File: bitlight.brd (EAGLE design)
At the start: 50.8 x 33 mm, 34 parts, among them Q1 SI4126DY-T1-GE3, Q2 FDC6330L, U1 TLV521DCKT, U2 NCP500SN33, U3 MCP73833

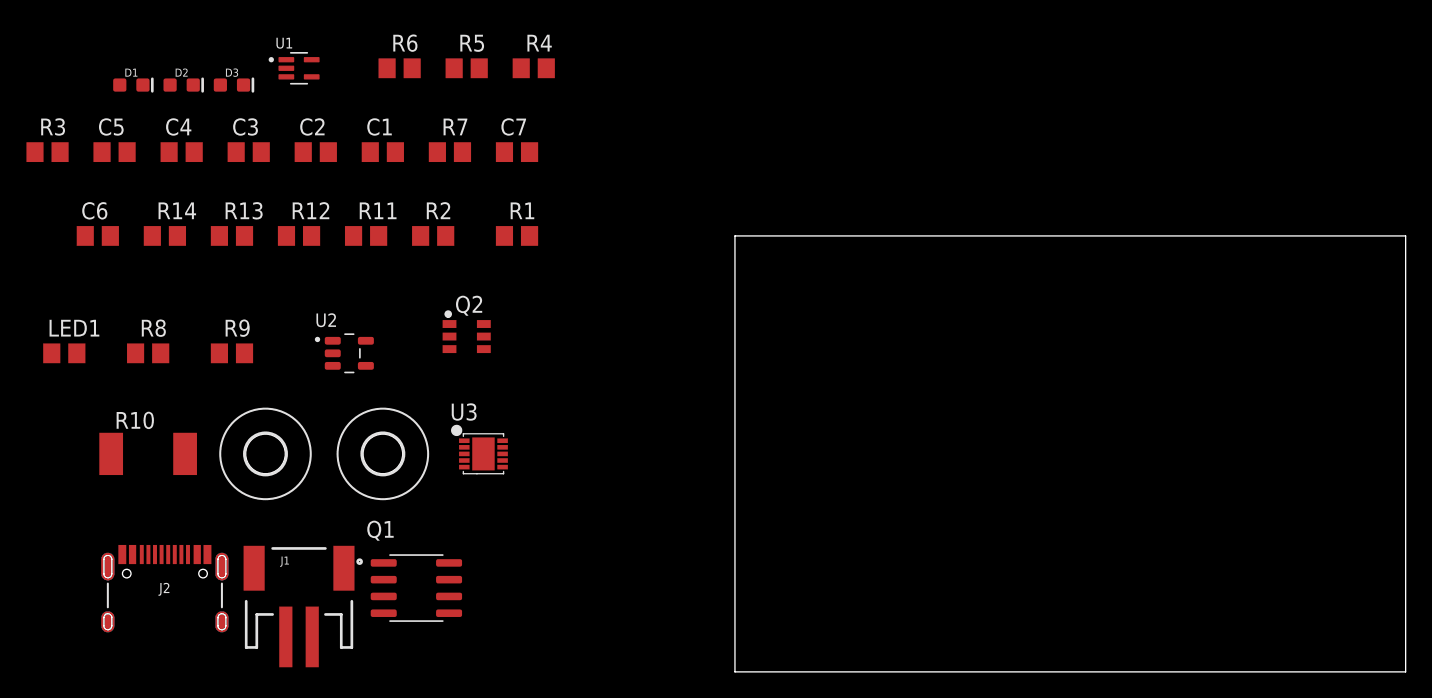
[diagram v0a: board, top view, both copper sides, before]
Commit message: final design
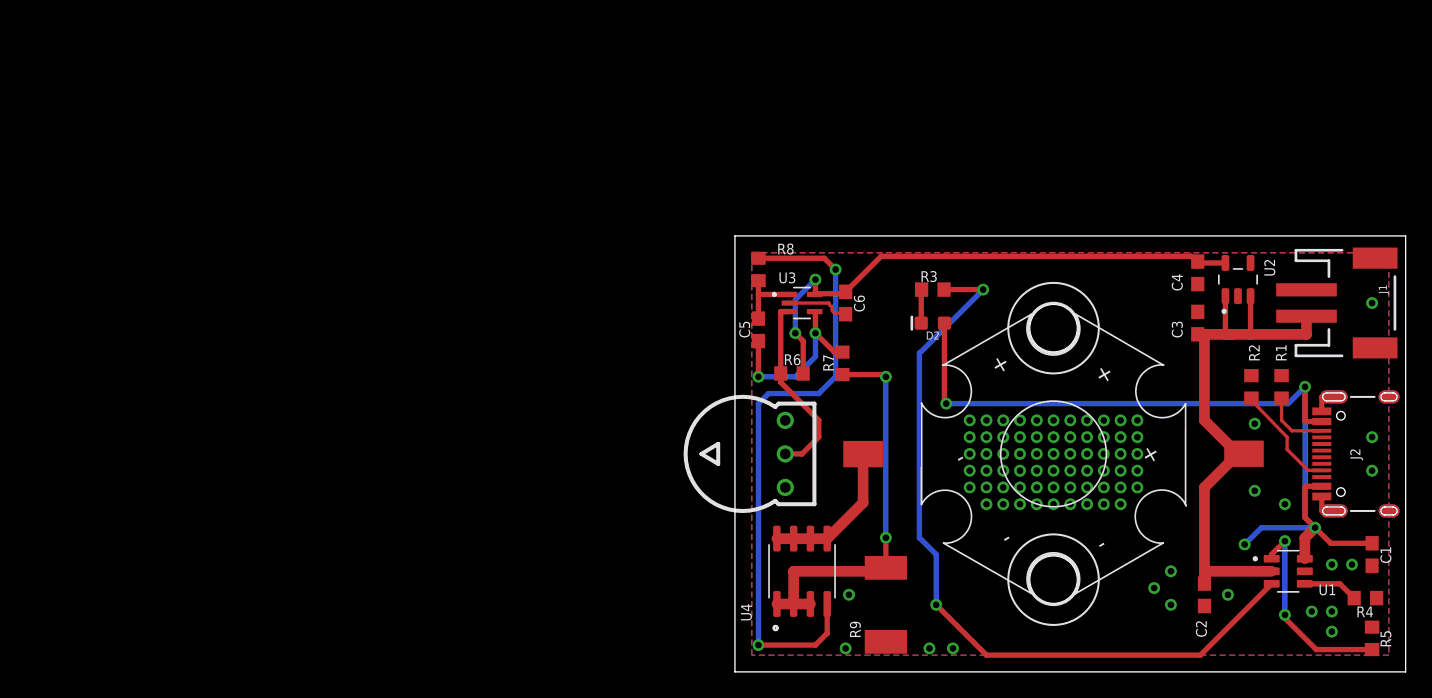
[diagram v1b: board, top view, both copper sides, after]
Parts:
- removed C7: 0.1u, rcl:C0805
- removed D3: Yellow, SparkFun-LED:LED-0603
- removed LED1: LED, rcl:C0805
- removed Q1: SI4126DY-T1-GE3, SI4126DY-T1-GE3:SOIC127P600X175-8N
- removed Q2: FDC6330L, FDC6330L:SOT95P280X110-6N
- removed R10: 0.5, rcl:R2512
- removed R11, R12, R14: 1k, rcl:R0805
- removed R13: 10k, rcl:R0805
- added P1: 3352T-1-105, 3352T-1:3352T-1
- added U4: SI4126DY-T1-GE3, SI4126DY-T1-GE3:SOIC127P600X175-8N
- C1, C2, C3, C4, C6: device rcl:C0805 -> rcl:C0603
- C5: value 1n -> 0.1u; device rcl:C0805 -> rcl:C0603
- D1: value RED -> 3W-AL-PCB; device SparkFun-LED:LED-0603 -> 3W-AL-PCB:AL-PCB-20MM
- H1, H2: value MOUNT-HOLE3.0 -> MOUNT-HOLE3.6; device holes:3,0 -> holes:3,6
- R1, R2, R3: device rcl:R0805 -> rcl:R0603
- R4: value 1k -> 680; device rcl:R0805 -> rcl:R0603
- R5: value 1k -> 10k; device rcl:R0805 -> rcl:R0603
- R6: value 1k -> 7.5M; device rcl:R0805 -> rcl:R0603
- R7: value 10k -> 1k; device rcl:R0805 -> rcl:R0603
- R8: value 7.5M -> 1k; device rcl:R0805 -> rcl:R0603
- R9: value 1M-pot -> 0.5; device rcl:R0805 -> rcl:R2512
- U1: value TLV521DCKT -> BQ21040DBVT; device TLV521DCKT:SOT65P210X110-5N -> BQ21040DBVT:SOT95P280X145-6N
- U3: value MCP73833 -> TLV521DCKT; device SparkFun-IC-Power:DFN-10 -> TLV521DCKT:SOT65P210X110-5N
- moved J2 88.0 mm to (44.5, 16.5), turned to 90 degrees
- moved U1 84.1 mm to (41.9, 7.62)
- moved J1 82.9 mm to (47.0, 27.9), turned to 270 degrees
- moved R5 81.0 mm to (48.3, 2.54), turned to 270 degrees
- moved C1 80.9 mm to (48.3, 8.89), turned to 270 degrees
- moved C4 77.5 mm to (35.1, 30.2), turned to 270 degrees
- moved D1 75.2 mm to (24.1, 16.5), turned to 210 degrees
- moved C2 75.2 mm to (35.6, 5.84), turned to 270 degrees
- moved R4 74.7 mm to (47.8, 5.59), turned to 180 degrees
- moved C3 73.0 mm to (35.1, 26.4), turned to 90 degrees
- moved R3 67.9 mm to (15.0, 29.0)
- moved U2 67.5 mm to (38.1, 29.7), turned to 90 degrees
- moved R2 63.0 mm to (39.1, 21.6), turned to 270 degrees
- moved H2 60.4 mm to (24.1, 26.0)
- moved D2 59.7 mm to (15.0, 26.4), turned to 180 degrees
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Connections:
- removed net N$11: C2.1, Q2.4, R13.2, U3.P$10, U3.P$9
- removed net N$14: C5.2, Q2.6, R13.1
- removed net N$15: Q2.1, R14.2
- removed net N$4: D1.C, R5.1
- removed net N$6: D3.C, R3.1
- removed net PG: R5.2, U3.P$7
- removed net STAT1: R3.2, U3.P$3
- removed net STAT2: R4.2, U3.P$4
- new net N$12: P1.WIPE, R6.1, U3.3
- net +3V3: now also R6.2, U3.5; no longer R8.2, U1.5
- net +5V: now also U1.6; no longer D1.A, D3.A, Q2.5, U3.P$1, U3.P$2
- net GND: now also P1.CCW, R4.1, R5.1, U1.5, U3.2; no longer R10.1, R14.1, R6.1, R7.1, U1.2, U3.P$11, U3.P$5
- net N$1: now also R3.2, U1.3; no longer R8.1, R9.2
- net N$10: now also R8.1, U4.4; no longer Q1.4, R11.1
- net N$2: now also C5.1, R7.2, U3.4; no longer C7.1, R12.2, U1.4
- net N$3: now also D1.-, U4.5, U4.6, U4.7, U4.8; no longer LED1.2, Q1.5, Q1.6, Q1.7, Q1.8
- net N$5: now also R3.1; no longer R4.1
- net N$7: now also R7.1, R9.2, U4.1, U4.2, U4.3; no longer Q1.1, Q1.2, Q1.3, R10.2, R12.1
- net N$8: now also C5.2, R8.2, U3.1; no longer C7.2, R11.2, U1.1
- net PROG: now also R4.2, U1.4; no longer R6.2, U3.P$6
- net THERM: now also R5.2, U1.1; no longer R7.2, U3.P$8
- net V_BATT: now also C2.1, D1.+, U1.2; no longer C5.1, LED1.1, Q2.2, Q2.3
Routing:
- net +5V: track 0.00 -> 66.8 mm, vias 0 -> 4
- net N$1: track 0.00 -> 58.6 mm, vias 0 -> 2
- net N$10: track 0.00 -> 47.1 mm, vias 0 -> 2
- net V_BATT: track 0.00 -> 44.5 mm
- net +3V3: track 0.00 -> 41.7 mm, vias 0 -> 2
- net N$7: track 0.00 -> 30.0 mm, vias 0 -> 2
- net THERM: track 0.00 -> 15.2 mm, vias 0 -> 2
- net N$12: track 0.00 -> 14.4 mm
- net N$2: track 0.00 -> 13.7 mm, vias 0 -> 2
- net N$3: track 0.00 -> 11.3 mm
- net GND: track 0.00 -> 8.78 mm, vias 0 -> 83
- net N$13: track 0.00 -> 8.27 mm
- net N$8: track 0.00 -> 5.21 mm
- net N$9: track 0.00 -> 5.07 mm
- net PROG: track 0.00 -> 4.19 mm
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- added copper zone on layer 1, net GND
- added copper zone on layer 16, net GND
